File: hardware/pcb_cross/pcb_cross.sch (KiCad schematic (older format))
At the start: 7 parts, among them J1 C96ABC, J2 C96ABC, J3 C96ABC, J4 C96ABC, J5 C96ABC, J6 PWR1, J7 PWR2

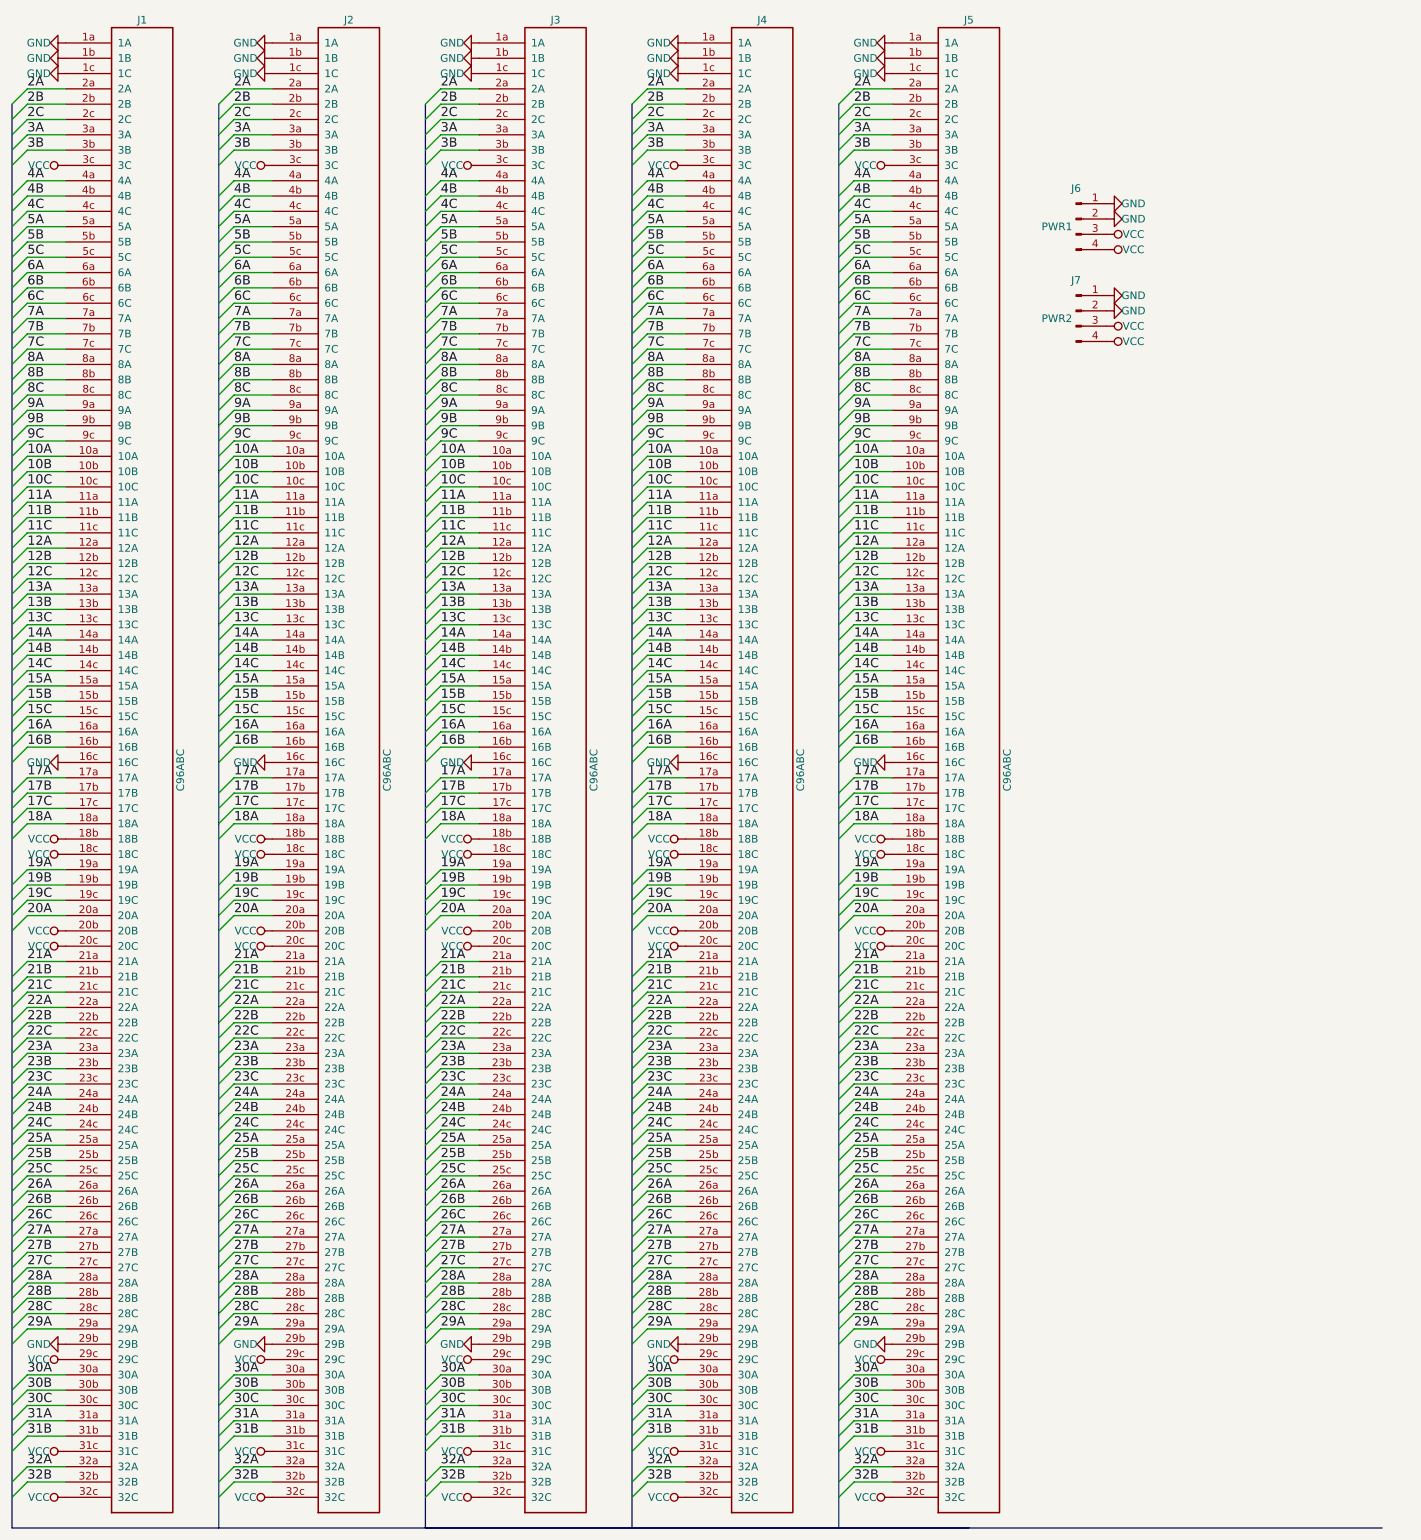
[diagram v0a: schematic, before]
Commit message: Актуализированна аппаратная часть
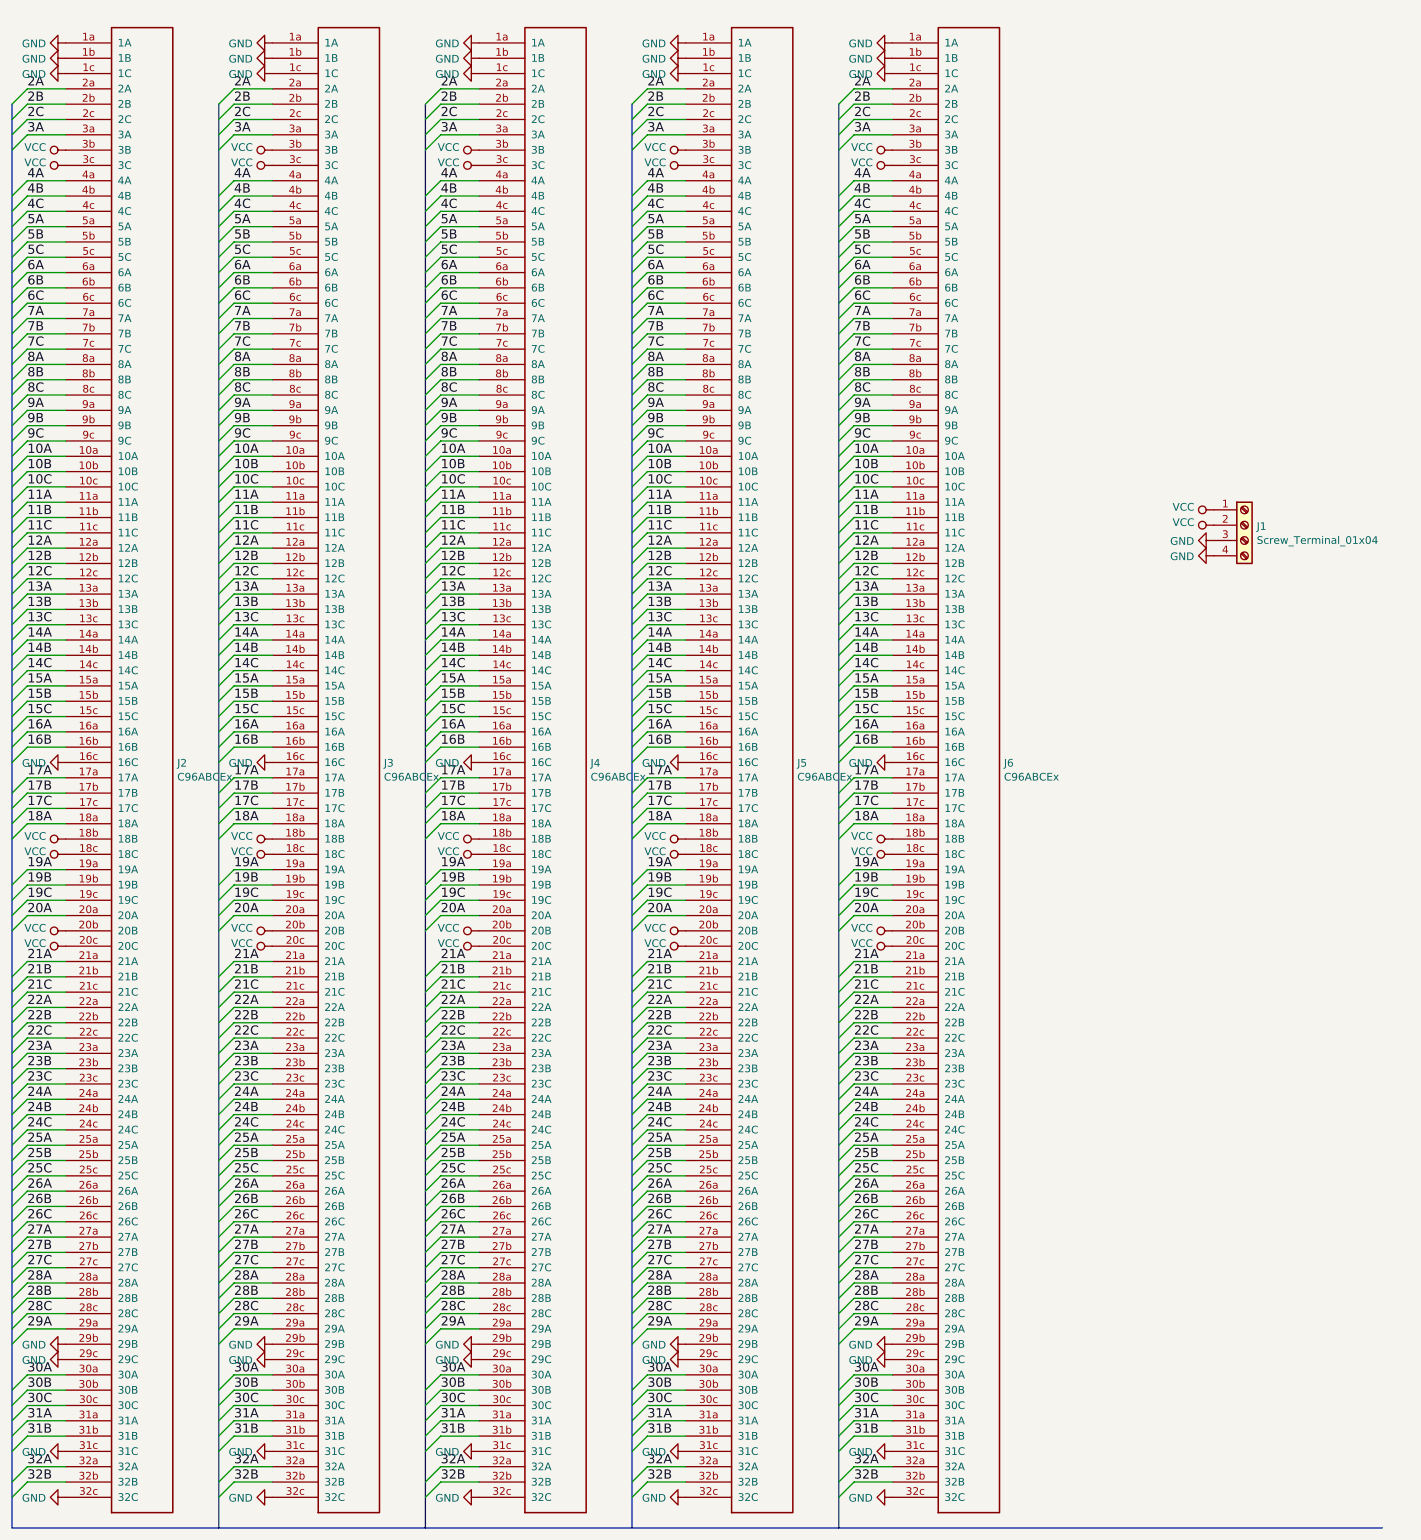
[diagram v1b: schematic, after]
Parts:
- removed J1, J2, J3, J4, J5: C96ABC, orion:Socket_DIN41612-CaseC1-full-Female-96Pin-3rows, symbol C96ABC-RESCUE-pcb_cross
- removed J6: PWR1, Connectors_Phoenix:PhoenixContact_MC-G_04x5.08mm_Angled, symbol Conn_01x04_Male
- removed J7: PWR2, Connectors_Phoenix:PhoenixContact_MC-G_04x5.08mm_Angled, symbol Conn_01x04_Male
- added J1: Screw_Terminal_01x04, Connector_Phoenix_MSTB:PhoenixContact_MSTBA_2,5_4-G_1x04_P5.00mm_Horizontal, symbol Connector:Screw_Terminal_01x04
- added J2, J3, J4, J5, J6: C96ABCEx, orion:Socket_DIN41612-CaseC1-full-Female-96Pin-3rows, symbol andreil:C96ABCEx
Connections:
- net 10A: now also J2.10a (10A), J3.10a (10A), J4.10a (10A), J5.10a (10A), J6.10a (10A)
- net 10B: now also J2.10b (10B), J3.10b (10B), J4.10b (10B), J5.10b (10B), J6.10b (10B)
- net 10C: now also J2.10c (10C), J3.10c (10C), J4.10c (10C), J5.10c (10C), J6.10c (10C)
- net 11A: now also J2.11a (11A), J3.11a (11A), J4.11a (11A), J5.11a (11A), J6.11a (11A)
- net 11B: now also J2.11b (11B), J3.11b (11B), J4.11b (11B), J5.11b (11B), J6.11b (11B)
- net 11C: now also J2.11c (11C), J3.11c (11C), J4.11c (11C), J5.11c (11C), J6.11c (11C)
- net 12A: now also J2.12a (12A), J3.12a (12A), J4.12a (12A), J5.12a (12A), J6.12a (12A)
- net 12B: now also J2.12b (12B), J3.12b (12B), J4.12b (12B), J5.12b (12B), J6.12b (12B)
- net 12C: now also J2.12c (12C), J3.12c (12C), J4.12c (12C), J5.12c (12C), J6.12c (12C)
- net 13A: now also J2.13a (13A), J3.13a (13A), J4.13a (13A), J5.13a (13A), J6.13a (13A)
- net 13B: now also J2.13b (13B), J3.13b (13B), J4.13b (13B), J5.13b (13B), J6.13b (13B)
- net 13C: now also J2.13c (13C), J3.13c (13C), J4.13c (13C), J5.13c (13C), J6.13c (13C)
- net 14A: now also J2.14a (14A), J3.14a (14A), J4.14a (14A), J5.14a (14A), J6.14a (14A)
- net 14B: now also J2.14b (14B), J3.14b (14B), J4.14b (14B), J5.14b (14B), J6.14b (14B)
- net 14C: now also J2.14c (14C), J3.14c (14C), J4.14c (14C), J5.14c (14C), J6.14c (14C)
- net 15A: now also J2.15a (15A), J3.15a (15A), J4.15a (15A), J5.15a (15A), J6.15a (15A)
- net 15B: now also J2.15b (15B), J3.15b (15B), J4.15b (15B), J5.15b (15B), J6.15b (15B)
- net 15C: now also J2.15c (15C), J3.15c (15C), J4.15c (15C), J5.15c (15C), J6.15c (15C)
- net 16A: now also J2.16a (16A), J3.16a (16A), J4.16a (16A), J5.16a (16A), J6.16a (16A)
- net 16B: now also J2.16b (16B), J3.16b (16B), J4.16b (16B), J5.16b (16B), J6.16b (16B)
- net 17A: now also J2.17a (17A), J3.17a (17A), J4.17a (17A), J5.17a (17A), J6.17a (17A)
- net 17B: now also J2.17b (17B), J3.17b (17B), J4.17b (17B), J5.17b (17B), J6.17b (17B)
- net 17C: now also J2.17c (17C), J3.17c (17C), J4.17c (17C), J5.17c (17C), J6.17c (17C)
- net 18A: now also J2.18a (18A), J3.18a (18A), J4.18a (18A), J5.18a (18A), J6.18a (18A)
- net 19A: now also J2.19a (19A), J3.19a (19A), J4.19a (19A), J5.19a (19A), J6.19a (19A)
- net 19B: now also J2.19b (19B), J3.19b (19B), J4.19b (19B), J5.19b (19B), J6.19b (19B)
- net 19C: now also J2.19c (19C), J3.19c (19C), J4.19c (19C), J5.19c (19C), J6.19c (19C)
- net 20A: now also J2.20a (20A), J3.20a (20A), J4.20a (20A), J5.20a (20A), J6.20a (20A)
- net 21A: now also J2.21a (21A), J3.21a (21A), J4.21a (21A), J5.21a (21A), J6.21a (21A)
- net 21B: now also J2.21b (21B), J3.21b (21B), J4.21b (21B), J5.21b (21B), J6.21b (21B)
- net 21C: now also J2.21c (21C), J3.21c (21C), J4.21c (21C), J5.21c (21C), J6.21c (21C)
- net 22A: now also J2.22a (22A), J3.22a (22A), J4.22a (22A), J5.22a (22A), J6.22a (22A)
- net 22B: now also J2.22b (22B), J3.22b (22B), J4.22b (22B), J5.22b (22B), J6.22b (22B)
- net 22C: now also J2.22c (22C), J3.22c (22C), J4.22c (22C), J5.22c (22C), J6.22c (22C)
- net 23A: now also J2.23a (23A), J3.23a (23A), J4.23a (23A), J5.23a (23A), J6.23a (23A)
- net 23B: now also J2.23b (23B), J3.23b (23B), J4.23b (23B), J5.23b (23B), J6.23b (23B)
- net 23C: now also J2.23c (23C), J3.23c (23C), J4.23c (23C), J5.23c (23C), J6.23c (23C)
- net 24A: now also J2.24a (24A), J3.24a (24A), J4.24a (24A), J5.24a (24A), J6.24a (24A)
- net 24B: now also J2.24b (24B), J3.24b (24B), J4.24b (24B), J5.24b (24B), J6.24b (24B)
- net 24C: now also J2.24c (24C), J3.24c (24C), J4.24c (24C), J5.24c (24C), J6.24c (24C)
- net 25A: now also J2.25a (25A), J3.25a (25A), J4.25a (25A), J5.25a (25A), J6.25a (25A)
- net 25B: now also J2.25b (25B), J3.25b (25B), J4.25b (25B), J5.25b (25B), J6.25b (25B)
- net 25C: now also J2.25c (25C), J3.25c (25C), J4.25c (25C), J5.25c (25C), J6.25c (25C)
- net 26A: now also J2.26a (26A), J3.26a (26A), J4.26a (26A), J5.26a (26A), J6.26a (26A)
- net 26B: now also J2.26b (26B), J3.26b (26B), J4.26b (26B), J5.26b (26B), J6.26b (26B)
- net 26C: now also J2.26c (26C), J3.26c (26C), J4.26c (26C), J5.26c (26C), J6.26c (26C)
- net 27A: now also J2.27a (27A), J3.27a (27A), J4.27a (27A), J5.27a (27A), J6.27a (27A)
- net 27B: now also J2.27b (27B), J3.27b (27B), J4.27b (27B), J5.27b (27B), J6.27b (27B)
- net 27C: now also J2.27c (27C), J3.27c (27C), J4.27c (27C), J5.27c (27C), J6.27c (27C)
- net 28A: now also J2.28a (28A), J3.28a (28A), J4.28a (28A), J5.28a (28A), J6.28a (28A)
- net 28B: now also J2.28b (28B), J3.28b (28B), J4.28b (28B), J5.28b (28B), J6.28b (28B)
- net 28C: now also J2.28c (28C), J3.28c (28C), J4.28c (28C), J5.28c (28C), J6.28c (28C)
- net 29A: now also J2.29a (29A), J3.29a (29A), J4.29a (29A), J5.29a (29A), J6.29a (29A)
- net 2A: now also J2.2a (2A), J3.2a (2A), J4.2a (2A), J5.2a (2A), J6.2a (2A)
- net 2B: now also J2.2b (2B), J3.2b (2B), J4.2b (2B), J5.2b (2B), J6.2b (2B)
- net 2C: now also J2.2c (2C), J3.2c (2C), J4.2c (2C), J5.2c (2C), J6.2c (2C)
- net 30A: now also J2.30a (30A), J3.30a (30A), J4.30a (30A), J5.30a (30A), J6.30a (30A)
- net 30B: now also J2.30b (30B), J3.30b (30B), J4.30b (30B), J5.30b (30B), J6.30b (30B)
- net 30C: now also J2.30c (30C), J3.30c (30C), J4.30c (30C), J5.30c (30C), J6.30c (30C)
- net 31A: now also J2.31a (31A), J3.31a (31A), J4.31a (31A), J5.31a (31A), J6.31a (31A)
- net 31B: now also J2.31b (31B), J3.31b (31B), J4.31b (31B), J5.31b (31B), J6.31b (31B)
- net 32A: now also J2.32a (32A), J3.32a (32A), J4.32a (32A), J5.32a (32A), J6.32a (32A)
- net 32B: now also J2.32b (32B), J3.32b (32B), J4.32b (32B), J5.32b (32B), J6.32b (32B)
- net 3A: now also J2.3a (3A), J3.3a (3A), J4.3a (3A), J5.3a (3A), J6.3a (3A)
- net 4A: now also J2.4a (4A), J3.4a (4A), J4.4a (4A), J5.4a (4A), J6.4a (4A)
- net 4B: now also J2.4b (4B), J3.4b (4B), J4.4b (4B), J5.4b (4B), J6.4b (4B)
- net 4C: now also J2.4c (4C), J3.4c (4C), J4.4c (4C), J5.4c (4C), J6.4c (4C)
- net 5A: now also J2.5a (5A), J3.5a (5A), J4.5a (5A), J5.5a (5A), J6.5a (5A)
- net 5B: now also J2.5b (5B), J3.5b (5B), J4.5b (5B), J5.5b (5B), J6.5b (5B)
- net 5C: now also J2.5c (5C), J3.5c (5C), J4.5c (5C), J5.5c (5C), J6.5c (5C)
- net 6A: now also J2.6a (6A), J3.6a (6A), J4.6a (6A), J5.6a (6A), J6.6a (6A)
- net 6B: now also J2.6b (6B), J3.6b (6B), J4.6b (6B), J5.6b (6B), J6.6b (6B)
- net 6C: now also J2.6c (6C), J3.6c (6C), J4.6c (6C), J5.6c (6C), J6.6c (6C)
- net 7A: now also J2.7a (7A), J3.7a (7A), J4.7a (7A), J5.7a (7A), J6.7a (7A)
- net 7B: now also J2.7b (7B), J3.7b (7B), J4.7b (7B), J5.7b (7B), J6.7b (7B)
- net 7C: now also J2.7c (7C), J3.7c (7C), J4.7c (7C), J5.7c (7C), J6.7c (7C)
- net 8A: now also J2.8a (8A), J3.8a (8A), J4.8a (8A), J5.8a (8A), J6.8a (8A)
- net 8B: now also J2.8b (8B), J3.8b (8B), J4.8b (8B), J5.8b (8B), J6.8b (8B)
- net 8C: now also J2.8c (8C), J3.8c (8C), J4.8c (8C), J5.8c (8C), J6.8c (8C)
- net 9A: now also J2.9a (9A), J3.9a (9A), J4.9a (9A), J5.9a (9A), J6.9a (9A)
- net 9B: now also J2.9b (9B), J3.9b (9B), J4.9b (9B), J5.9b (9B), J6.9b (9B)
- net 9C: now also J2.9c (9C), J3.9c (9C), J4.9c (9C), J5.9c (9C), J6.9c (9C)
- net GND: now also J1.3 (Pin_3), J1.4 (Pin_4), J2.16c (16C), J2.1a (1A), J2.1b (1B), J2.1c (1C), J2.29b (29B), J2.29c (29C), J2.31c (31C), J2.32c (32C), J3.16c (16C), J3.1a (1A), J3.1b (1B), J3.1c (1C), J3.29b (29B), J3.29c (29C), J3.31c (31C), J3.32c (32C), J4.16c (16C), J4.1a (1A), J4.1b (1B), J4.1c (1C), J4.29b (29B), J4.29c (29C), J4.31c (31C), J4.32c (32C), J5.16c (16C), J5.1a (1A), J5.1b (1B), J5.1c (1C), J5.29b (29B), J5.29c (29C), J5.31c (31C), J5.32c (32C), J6.16c (16C), J6.1a (1A), J6.1b (1B), J6.1c (1C), J6.29b (29B), J6.29c (29C), J6.31c (31C), J6.32c (32C)
- net VCC: now also J1.1 (Pin_1), J1.2 (Pin_2), J2.18b (18B), J2.18c (18C), J2.20b (20B), J2.20c (20C), J2.3b (3B), J2.3c (3C), J3.18b (18B), J3.18c (18C), J3.20b (20B), J3.20c (20C), J3.3b (3B), J3.3c (3C), J4.18b (18B), J4.18c (18C), J4.20b (20B), J4.20c (20C), J4.3b (3B), J4.3c (3C), J5.18b (18B), J5.18c (18C), J5.20b (20B), J5.20c (20C), J5.3b (3B), J5.3c (3C), J6.18b (18B), J6.18c (18C), J6.20b (20B), J6.20c (20C), J6.3b (3B), J6.3c (3C)
